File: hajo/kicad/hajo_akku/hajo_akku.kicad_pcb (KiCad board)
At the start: 2 copper layers, 68.6 x 73.7 mm, 18 parts, among them J1 Seetalk NG, J2 Batteries, J4 Device type, U1 MCP2562, U2 LF50CV

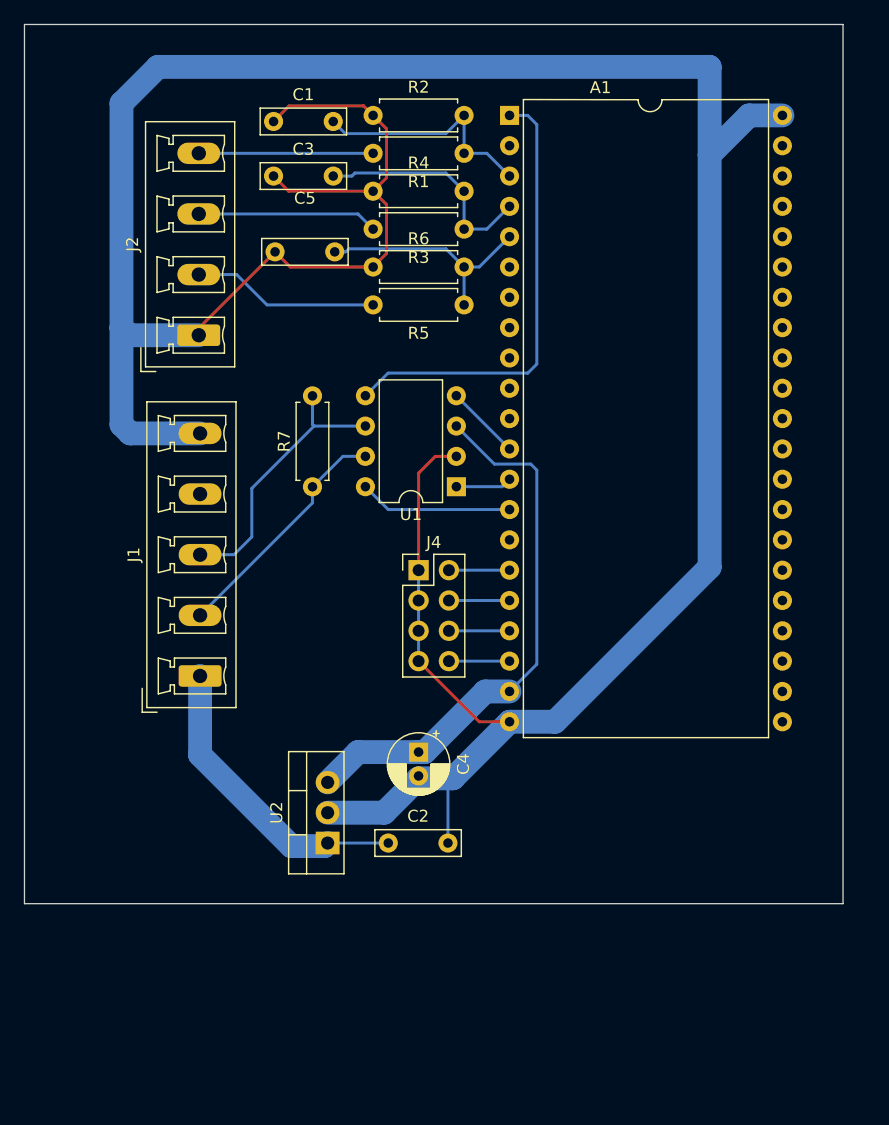
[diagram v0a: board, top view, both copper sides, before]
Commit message: final pcb
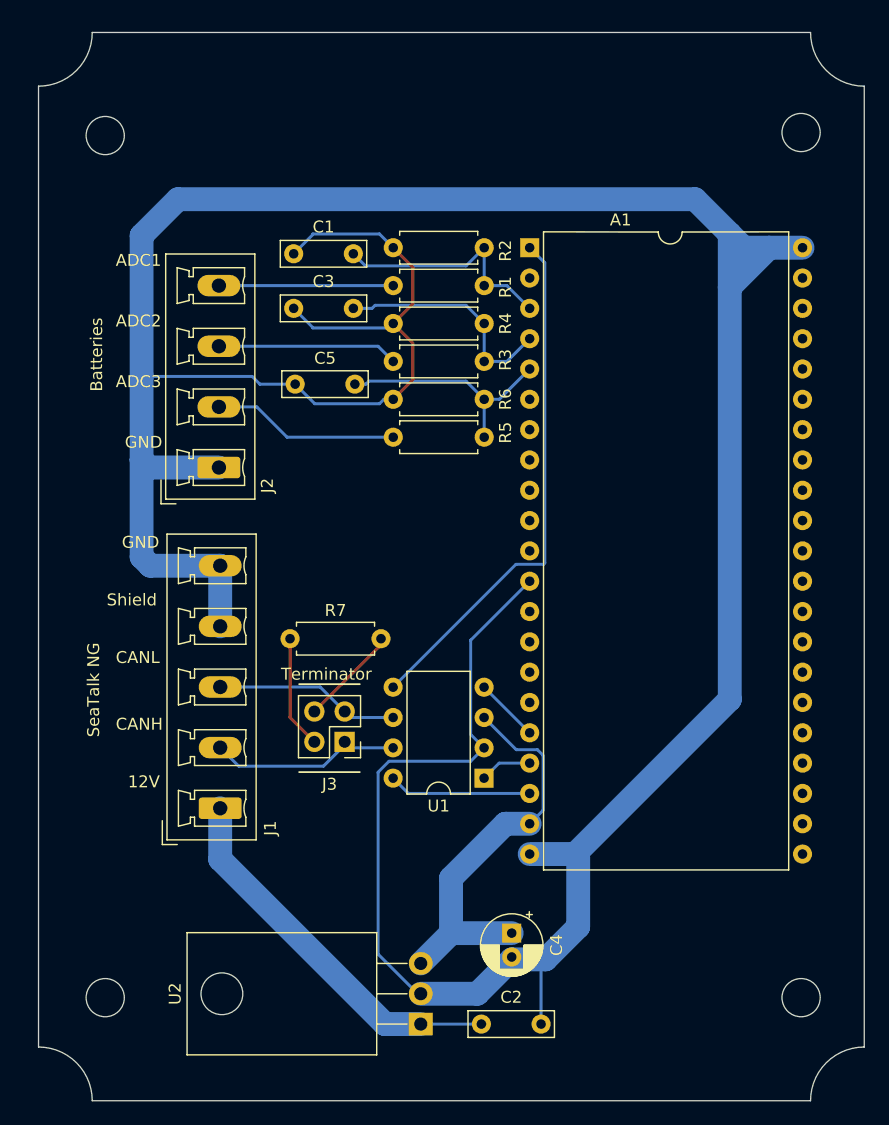
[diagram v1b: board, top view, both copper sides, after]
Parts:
- removed J4: Device type, Connector_PinHeader_2.54mm:PinHeader_2x04_P2.54mm_Vertical
- added H1: MountingHole, MountingHole:MountingHole_3.2mm_M3, F.Cu at (76.9, 21.4)
- added H2: MountingHole, MountingHole:MountingHole_3.2mm_M3, F.Cu at (18.6, 93.9)
- added H3: MountingHole, MountingHole:MountingHole_3.2mm_M3, F.Cu at (18.6, 21.6)
- added H4: MountingHole, MountingHole:MountingHole_3.2mm_M3, F.Cu at (76.9, 93.9)
- added J3: Terminator, Connector_PinHeader_2.54mm:PinHeader_2x02_P2.54mm_Vertical, F.Cu at (38.6, 72.4)
- U2: footprint Package_TO_SOT_THT:TO-220-3_Vertical -> Package_TO_SOT_THT:TO-220-3_Horizontal_TabDown
- moved U1 24.5 mm to (50.3, 75.5)
- moved C4 17.1 mm to (52.6, 88.5)
- moved U2 17.1 mm to (45.0, 96.1)
- moved C2 17.1 mm to (50.1, 96.1)
- moved R7 12.9 mm to (34.1, 63.8), turned to 0 degrees
- moved J1 11.2 mm to (28.2, 78.0)
- moved J2 11.2 mm to (28.1, 49.4)
- moved R4 11.2 mm to (42.7, 37.4)
- moved R5 11.2 mm to (50.3, 46.9)
- moved A1 11.2 mm to (54.1, 31.0)
- moved C1 11.2 mm to (34.4, 31.5)
- moved C3 11.2 mm to (34.4, 36.1)
- moved C5 11.2 mm to (34.5, 42.5)
- moved R1 11.2 mm to (50.3, 34.2)
- moved R2 11.2 mm to (42.7, 31.0)
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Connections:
- A1 pad 12: /RXD -> GND
- A1 pad 13: /TXD -> unconnected-(A1-GPIO11/ADC2_0-Pad13)
- A1 pad 14: /STBY -> unconnected-(A1-GPIO12/ADC2_1-Pad14)
- A1 pad 16: Net-(A1-GPIO14/ADC2_3) -> unconnected-(A1-GPIO14/ADC2_3-Pad16)
- A1 pad 17: Net-(A1-GPIO15/ADC2_4/U0RTS) -> /RXD
- A1 pad 18: Net-(A1-GPIO16/ADC2_5/U0CTS) -> /TXD
- A1 pad 19: Net-(A1-GPIO17/ADC2_6/U1TXD) -> /STBY
- J1 pad 4: unconnected-(J1-Pin_4-Pad4) -> GND
- R7 pad 1: /CANH -> Net-(J3-Pin_2)
- R7 pad 2: /CANL -> Net-(J3-Pin_4)
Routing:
- net GND: track 266.8 -> 299.8 mm
- net +5V: track 46.2 -> 34.2 mm
- net Net-(J3-Pin_2): track 0.00 -> 9.48 mm
- net Net-(J3-Pin_4): track 0.00 -> 8.41 mm
- net /CANL: track 23.3 -> 15.5 mm
- net +12V: track 25.6 -> 31.9 mm
- net +3.3V: track 38.1 -> 44.0 mm
- net Net-(A1-GPIO17/ADC2_6/U1TXD): track 5.08 -> 0.00 mm
- net Net-(A1-GPIO16/ADC2_5/U0CTS): track 5.08 -> 0.00 mm
- net Net-(A1-GPIO15/ADC2_4/U0RTS): track 5.08 -> 0.00 mm
- net Net-(A1-GPIO14/ADC2_3): track 5.08 -> 0.00 mm
- net /CANH: track 20.2 -> 16.3 mm
- net /RXD: track 6.30 -> 5.40 mm
- net /STBY: track 12.9 -> 12.0 mm
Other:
- board size 68.6 x 73.7 mm -> 69.2 x 89.5 mm
- board text added: "12V"
- board text added: "ADC1"
- board text added: "ADC2"
- board text added: "ADC3"
- board text added: "Batteries"
- board text added: "CANH"
- board text added: "CANL"
- board text added: "GND"
- board text added: "SeaTalk NG"
- board text added: "Shield"
- board text added: "Terminator"
